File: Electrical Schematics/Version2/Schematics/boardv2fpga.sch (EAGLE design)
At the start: 159 parts, among them Q1 ASFL1

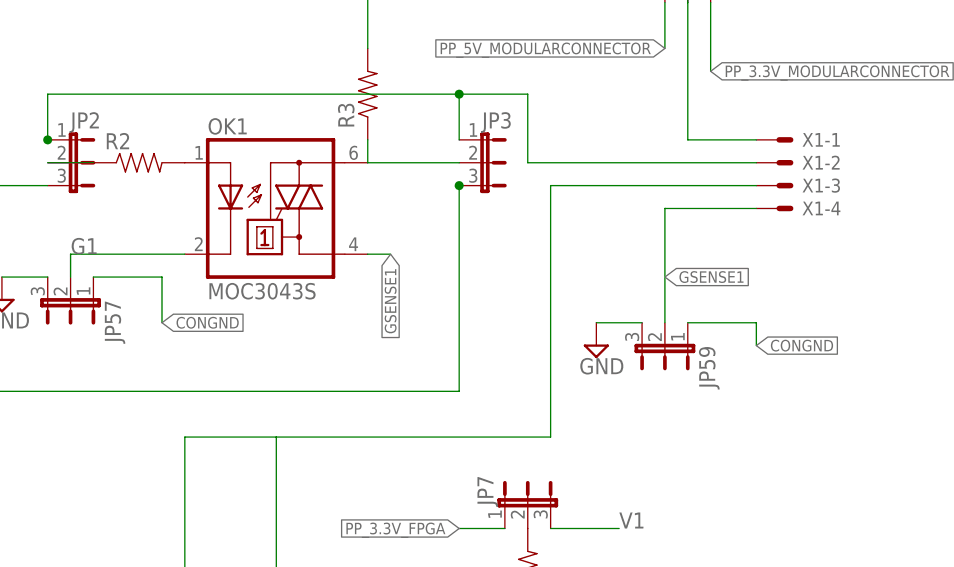
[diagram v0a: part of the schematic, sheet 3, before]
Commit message: updated circuits
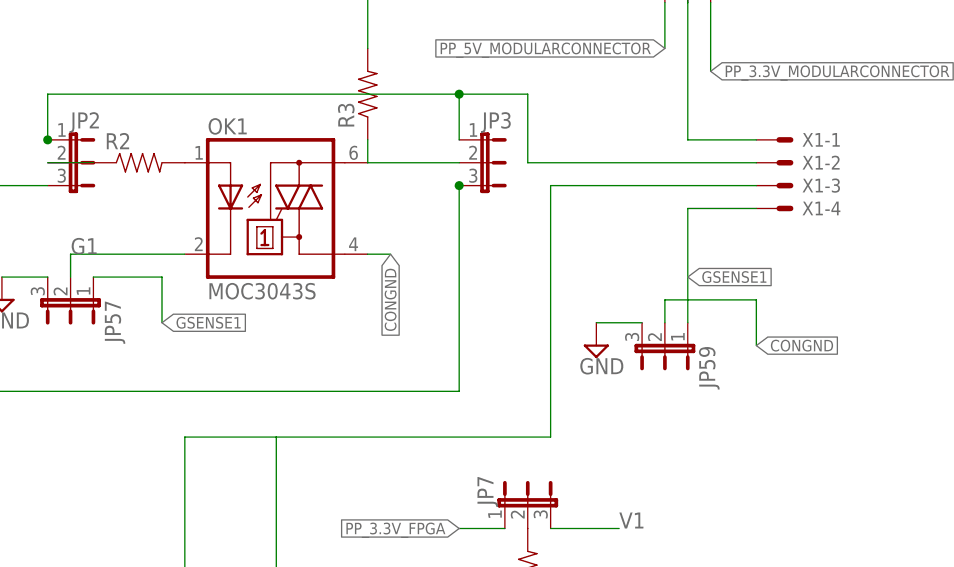
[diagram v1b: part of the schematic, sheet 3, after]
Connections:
- net CONGND: now also JP59.2, OK1.A1; no longer JP57.1, JP59.1
- net GSENSE1: now also JP57.1, JP59.1; no longer JP59.2, OK1.A1
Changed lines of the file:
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@@
 <setting verticaltext="up"/>
 </settings>
-<grid distance="0.1" unitdist="inch" unit="inch" style="lines" multiple="1" display="no" altdistance="0.05" altunitdist="inch" altunit="inch"/>
+<grid distance="0.1" unitdist="inch" unit="inch" style="lines" multiple="1" display="no" altdistance="0.01" altunitdist="inch" altunit="inch"/>
 <layers>
 <layer number="1" name="Top" color="4" fill="1" visible="no" active="no"/>
@@
 <net name="CONGND" class="0">
 <segment>
+<label x="68.58" y="48.26" size="1.27" layer="95" xref="yes"/>
+<wire x1="68.58" y1="48.26" x2="68.58" y2="53.34" width="0.1524" layer="91"/>
+<pinref part="JP59" gate="1" pin="2"/>
+<wire x1="68.58" y1="53.34" x2="58.42" y2="53.34" width="0.1524" layer="91"/>
+<wire x1="58.42" y1="53.34" x2="58.42" y2="50.8" width="0.1524" layer="91"/>
+</segment>
+<segment>
+<pinref part="OK1" gate="-1" pin="A1"/>
+<wire x1="25.4" y1="58.42" x2="27.94" y2="58.42" width="0.1524" layer="91"/>
+<label x="27.94" y="58.42" size="1.27" layer="95" rot="R270" xref="yes"/>
+</segment>
+</net>
+<net name="GSENSE1" class="0">
+<segment>
+<pinref part="OK2" gate="-1" pin="A1"/>
+<wire x1="40.64" y1="7.62" x2="43.18" y2="7.62" width="0.1524" layer="91"/>
+<label x="43.18" y="7.62" size="1.27" layer="95" rot="R270" xref="yes"/>
+</segment>
+<segment>
+<pinref part="X1" gate="-4" pin="S"/>
+<wire x1="68.58" y1="63.5" x2="60.96" y2="63.5" width="0.1524" layer="91"/>
+<label x="60.96" y="55.88" size="1.27" layer="95" xref="yes"/>
+<pinref part="JP59" gate="1" pin="1"/>
+<wire x1="60.96" y1="50.8" x2="60.96" y2="63.5" width="0.1524" layer="91"/>
+</segment>
+<segment>
 <pinref part="JP57" gate="1" pin="1"/>
 <wire x1="-5.08" y1="55.88" x2="2.54" y2="55.88" width="0.1524" layer="91"/>
@@
 <wire x1="2.54" y1="55.88" x2="2.54" y2="50.8" width="0.1524" layer="91"/>
 </segment>
-<segment>
-<pinref part="JP59" gate="1" pin="1"/>
-<wire x1="60.96" y1="50.8" x2="68.58" y2="50.8" width="0.1524" layer="91"/>
-<wire x1="68.58" y1="50.8" x2="68.58" y2="48.26" width="0.1524" layer="91"/>
-<label x="68.58" y="48.26" size="1.27" layer="95" xref="yes"/>
-</segment>
-</net>
-<net name="GSENSE1" class="0">
-<segment>
-<pinref part="OK2" gate="-1" pin="A1"/>
-<wire x1="40.64" y1="7.62" x2="43.18" y2="7.62" width="0.1524" layer="91"/>
-<label x="43.18" y="7.62" size="1.27" layer="95" rot="R270" xref="yes"/>
-</segment>
-<segment>
-<pinref part="X1" gate="-4" pin="S"/>
-<wire x1="68.58" y1="63.5" x2="58.42" y2="63.5" width="0.1524" layer="91"/>
-<pinref part="JP59" gate="1" pin="2"/>
-<wire x1="58.42" y1="63.5" x2="58.42" y2="50.8" width="0.1524" layer="91"/>
-<label x="58.42" y="55.88" size="1.27" layer="95" xref="yes"/>
-</segment>
-<segment>
-<pinref part="OK1" gate="-1" pin="A1"/>
-<wire x1="25.4" y1="58.42" x2="27.94" y2="58.42" width="0.1524" layer="91"/>
-<label x="27.94" y="58.42" size="1.27" layer="95" rot="R270" xref="yes"/>
-</segment>
-</net>
+</net>
